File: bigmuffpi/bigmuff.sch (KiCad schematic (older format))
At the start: 62 parts, among them J1 PWR JACK, J2 INPUT, J3 OUTPUT, Q1 BC239, Q2 BC239, Q3 BC239, Q4 BC239, SW1 POWER

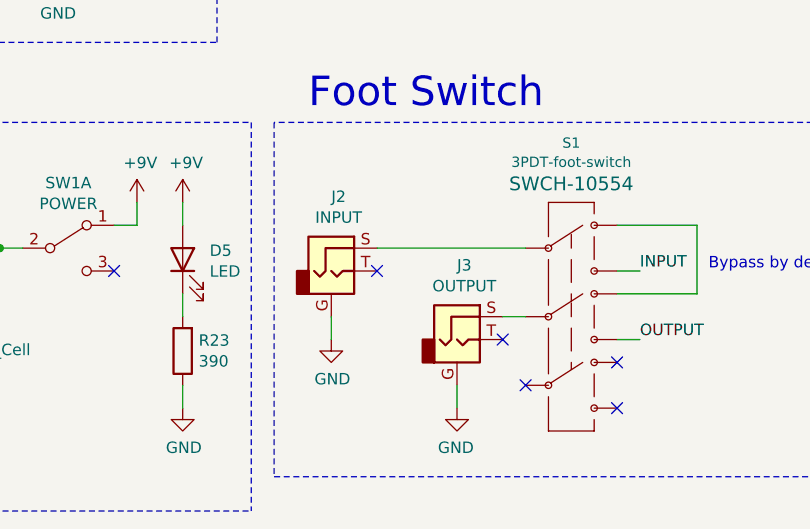
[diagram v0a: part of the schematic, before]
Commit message: add: mostly hw layout
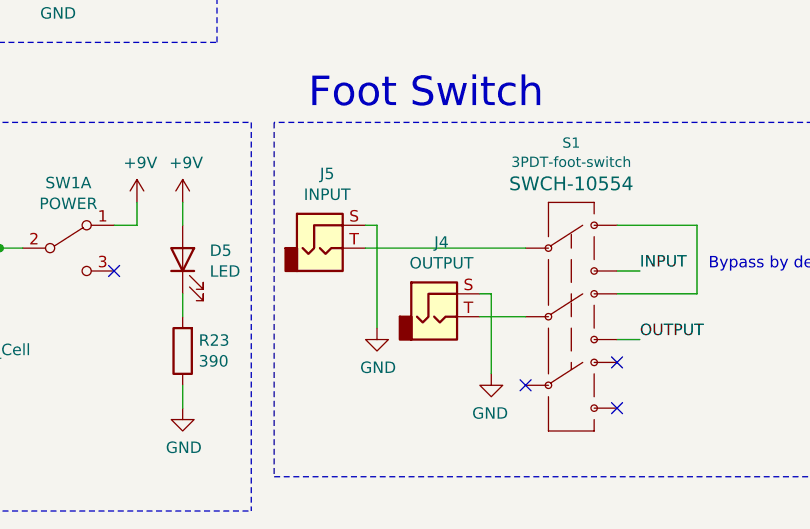
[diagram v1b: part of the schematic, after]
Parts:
- removed J2: INPUT, symbol Connector:AudioJack2_Ground
- removed J3: OUTPUT, symbol Connector:AudioJack2_Ground
- added J4: OUTPUT, bigmuffpi:NMJ6HC-S, symbol Connector:AudioJack2
- added J5: INPUT, bigmuffpi:NMJ6HC-S, symbol Connector:AudioJack2
- BT1: footprint (none) -> LED_THT:LED_D5.0mm; Mfr. No 232 -> 79; Mouser 534-232 -> 534-079
- C1, C5, C8: footprint Capacitor_THT:C_Disc_D5.0mm_W2.5mm_P5.00mm -> Capacitor_THT:CP_Radial_D5.0mm_P2.00mm
- C10, C11, C12, C13, C2, C3, C4, C6, C7, C9: footprint Capacitor_THT:C_Disc_D5.0mm_W2.5mm_P5.00mm -> Capacitor_THT:C_Disc_D4.7mm_W2.5mm_P5.00mm
- J1: footprint (none) -> Connector_PinHeader_2.54mm:PinHeader_1x03_P2.54mm_Vertical; LCSC C381116 -> (none); Mfr. No DC-005-5A-2.0 -> (none); Supplier LCSC -> Aliexpress
- S1: footprint (none) -> bigmuffpi:SF17020F-0302-21R-L
- SW1: footprint (none) -> bigmuffpi:E-SWITCH-100SP3T2B4M6RE
- Sustain1, Tone1, Volume1: footprint (none) -> Potentiometer_THT:Potentiometer_Alps_RK09K_Single_Vertical
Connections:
- net GND: now also J4.S, J5.S
- net at S1.2: now also J5.T
- net at S1.5: now also J4.T
- no-connect marks 6 -> 4
